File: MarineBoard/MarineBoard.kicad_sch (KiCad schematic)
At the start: 152 parts, among them CN1 MKDSN 1,5/ 2-5,08, CN2 MKDSN 1,5/ 2-5,08, CN3 SM04B-SRSS-TB (LF)(SN), J1 USB_C_Receptacle_USB2.0_16P, J3 Conn_02x09_Top_Bottom, Q1 IPL60R075CFD7, Q2 S8050, Q3 S8050, U1 SY8089A1AAC, U10 PC817C-S, U11 SN65HVD230DR, U12 DB125-3.5-3P-GN-S, U13 DB125-3.5-3P-GN-S, U14 PC817C-S, U15 TC4427EPA, U16 PC817C-S, U17 PC817C-S, U18 INA226, U19 INA226, U2 INA226, U20 SMAJ6.8CA, U3 TPS5430DDA, U4 DB125-3.5-2P-GN-S, U5 DB125-3.5-2P-GN-S, U6 DB125-3.5-2P-GN-S, U7 DB125-3.5-3P-GN-S, U8 ESP32-S3-WROOM-2-N32R16V, U9 DB125-3.5-3P-GN-S

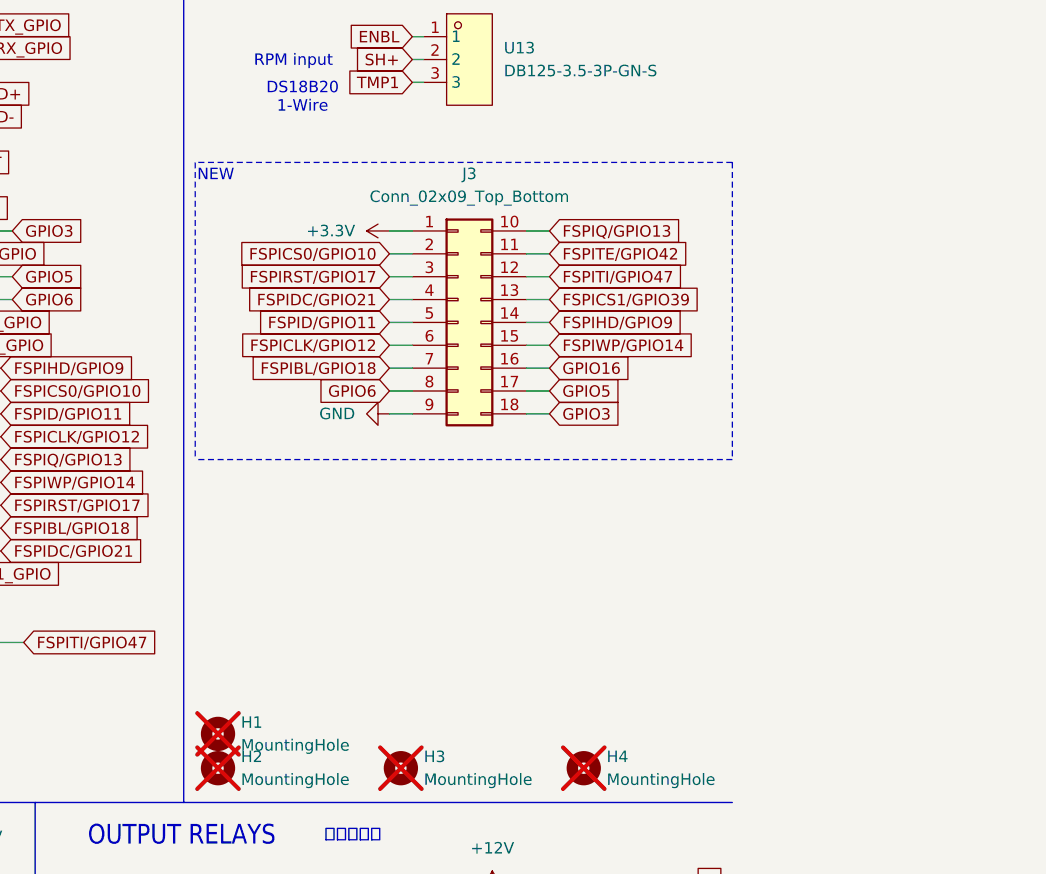
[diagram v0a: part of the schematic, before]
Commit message: MarineBoard: schematic library/component update
Co-Authored-By: Claude Sonnet 5 <noreply@anthropic.com>
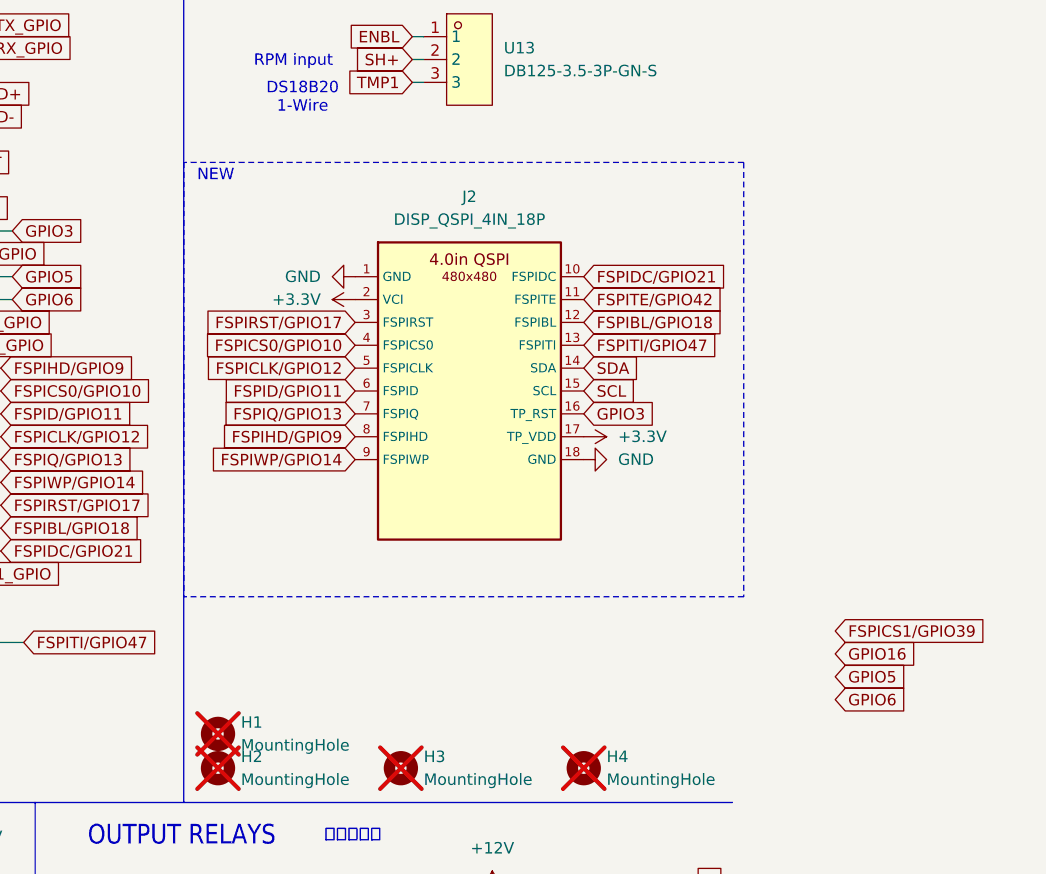
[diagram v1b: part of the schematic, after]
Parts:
- removed J3: Conn_02x09_Top_Bottom, Connector_PinHeader_1.27mm:PinHeader_2x09_P1.27mm_Vertical, symbol Connector_Generic:Conn_02x09_Top_Bottom
- added J2: DISP_QSPI_4IN_18P, EasyEDA:FH12-18S-0.5SH_QSPI4IN, symbol EasyEDA:DISP_QSPI_4IN_18P
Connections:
- net +3.3V: now also J2.17 (TP_VDD), J2.2 (VCI)
- net FSPIBL/GPIO18: now also J2.12 (FSPIBL)
- net FSPICLK/GPIO12: now also J2.5 (FSPICLK)
- net FSPICS0/GPIO10: now also J2.4 (FSPICS0)
- net FSPID/GPIO11: now also J2.6 (FSPID)
- net FSPIDC/GPIO21: now also J2.10 (FSPIDC)
- net FSPIHD/GPIO9: now also J2.8 (FSPIHD)
- net FSPIQ/GPIO13: now also J2.7 (FSPIQ)
- net FSPIRST/GPIO17: now also J2.3 (FSPIRST)
- net FSPITE/GPIO42: now also J2.11 (FSPITE)
- net FSPITI/GPIO47: now also J2.13 (FSPITI)
- net FSPIWP/GPIO14: now also J2.9 (FSPIWP)
- net GND: now also J2.1 (GND), J2.18 (GND)
- net GPIO3: now also J2.16 (TP_RST)
- net SCL: now also J2.15 (SCL)
- net SDA: now also J2.14 (SDA)
